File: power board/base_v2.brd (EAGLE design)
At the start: 60.4 x 36.6 mm, 59 parts, among them IC1 MCP2515-E/ST, Q2 QUARZ5, U1 INA209_PW_16, U2 LTC1540, U5 MSP430FR5739_DA_38, U6 SN65HVD235_D_8, X1 22-23-2021

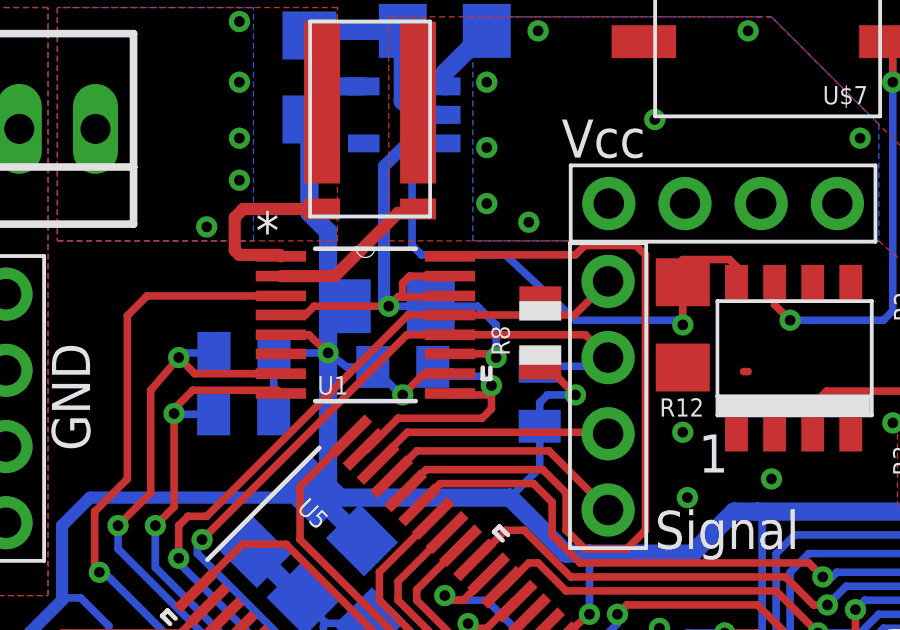
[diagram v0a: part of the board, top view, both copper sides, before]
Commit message: clean up schematics
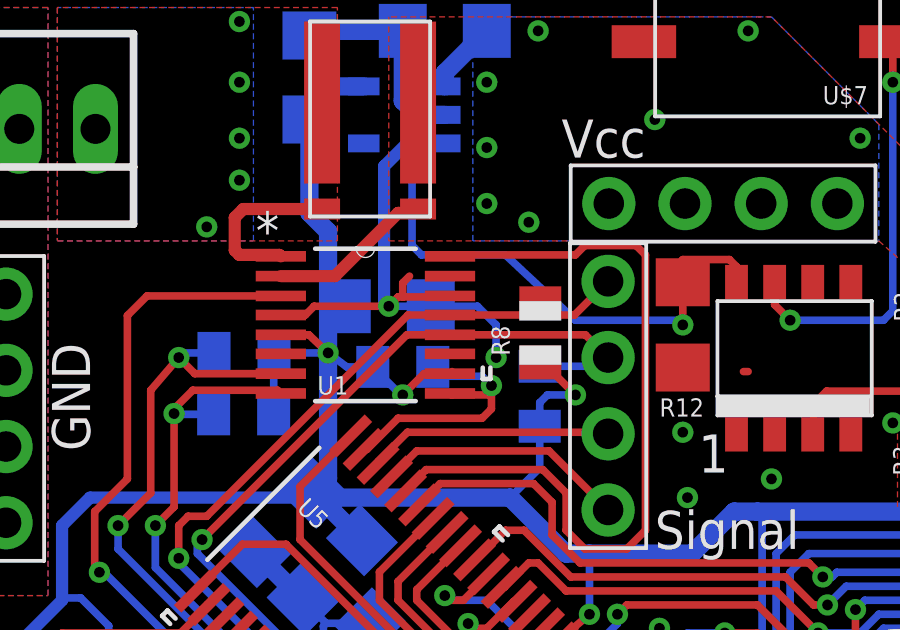
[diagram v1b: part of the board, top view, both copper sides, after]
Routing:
- net GND: track 86.9 -> 84.2 mm
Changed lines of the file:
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@@
 <layer number="39" name="tKeepout" color="4" fill="11" visible="yes" active="yes"/>
 <layer number="40" name="bKeepout" color="1" fill="11" visible="yes" active="yes"/>
-<layer number="41" name="tRestrict" color="4" fill="10" visible="yes" active="yes"/>
-<layer number="42" name="bRestrict" color="1" fill="10" visible="yes" active="yes"/>
+<layer number="41" name="tRestrict" color="4" fill="10" visible="no" active="yes"/>
+<layer number="42" name="bRestrict" color="1" fill="10" visible="no" active="yes"/>
 <layer number="43" name="vRestrict" color="2" fill="10" visible="yes" active="yes"/>
 <layer number="44" name="Drills" color="7" fill="1" visible="no" active="yes"/>
@@
 <layer number="46" name="Milling" color="3" fill="1" visible="no" active="yes"/>
 <layer number="47" name="Measures" color="7" fill="1" visible="no" active="yes"/>
-<layer number="48" name="Document" color="7" fill="1" visible="yes" active="yes"/>
-<layer number="49" name="Reference" color="7" fill="1" visible="yes" active="yes"/>
+<layer number="48" name="Document" color="7" fill="1" visible="no" active="yes"/>
+<layer number="49" name="Reference" color="7" fill="1" visible="no" active="yes"/>
 <layer number="50" name="dxf" color="7" fill="1" visible="no" active="no"/>
-<layer number="51" name="tDocu" color="7" fill="1" visible="yes" active="yes"/>
-<layer number="52" name="bDocu" color="7" fill="1" visible="yes" active="yes"/>
+<layer number="51" name="tDocu" color="7" fill="1" visible="no" active="yes"/>
+<layer number="52" name="bDocu" color="7" fill="1" visible="no" active="yes"/>
 <layer number="53" name="tGND_GNDA" color="7" fill="9" visible="no" active="no"/>
 <layer number="54" name="bGND_GNDA" color="1" fill="9" visible="no" active="no"/>
@@
 <wire x1="39.360475" y1="16.8021" x2="39.360475" y2="15.2175" width="0.254" layer="1"/>
 <wire x1="39.360475" y1="15.2175" x2="39.51605" y2="15.061925" width="0.254" layer="1"/>
-<contactref element="U1" pad="11"/>
-<contactref element="U1" pad="11"/>
-<contactref element="U1" pad="15"/>
-<contactref element="U1" pad="14"/>
 <contactref element="C11" pad="2"/>
 <contactref element="U1" pad="4"/>
-<contactref element="X1" pad="2"/>
 <contactref element="R12" pad="2"/>
 <contactref element="C13" pad="2"/>
@@
 <wire x1="14.9352" y1="20.691475" x2="15.090775" y2="20.691475" width="0.254" layer="1"/>
 <wire x1="15.090775" y1="20.691475" x2="16.633825" y2="20.691475" width="0.254" layer="1"/>
-<wire x1="16.633825" y1="20.691475" x2="16.665575" y2="20.723225" width="0.254" layer="1"/>
-<wire x1="16.665575" y1="21.383625" x2="15.3162" y2="21.383625" width="0.254" layer="1"/>
 <wire x1="15.3162" y1="21.383625" x2="15.090775" y2="21.1582" width="0.254" layer="1"/>
 <wire x1="11.026775" y1="20.088225" x2="11.84275" y2="20.088225" width="0.254" layer="1"/>
@@
 <wire x1="13.991734375" y1="9.81281875" x2="12.53826875" y2="9.81281875" width="0.254" layer="16"/>
 <wire x1="12.53826875" y1="9.81281875" x2="11.751490625" y2="10.599596875" width="0.254" layer="16"/>
-<wire x1="16.665575" y1="18.792825" x2="18.01495" y2="18.792825" width="0.254" layer="1"/>
 <wire x1="18.01495" y1="18.792825" x2="18.202275" y2="18.669" width="0.254" layer="1"/>
 <via x="18.202275" y="18.669" extent="1-16" drill="0.3556"/>
@@
 <vertex x="37.182425" y="22.558375"/>
 </polygon>
+<contactref element="U1" pad="11"/>
+<contactref element="U1" pad="11"/>
+<contactref element="U1" pad="15"/>
+<contactref element="U1" pad="14"/>
+<contactref element="X1" pad="2"/>
 </signal>
 <signal name="VCORE">
